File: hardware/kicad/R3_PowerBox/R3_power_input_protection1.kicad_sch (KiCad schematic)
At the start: 13 parts, among them J1 SERVICE / BENCH INPUT 6-12V, Q1 DMP3010LSS-13

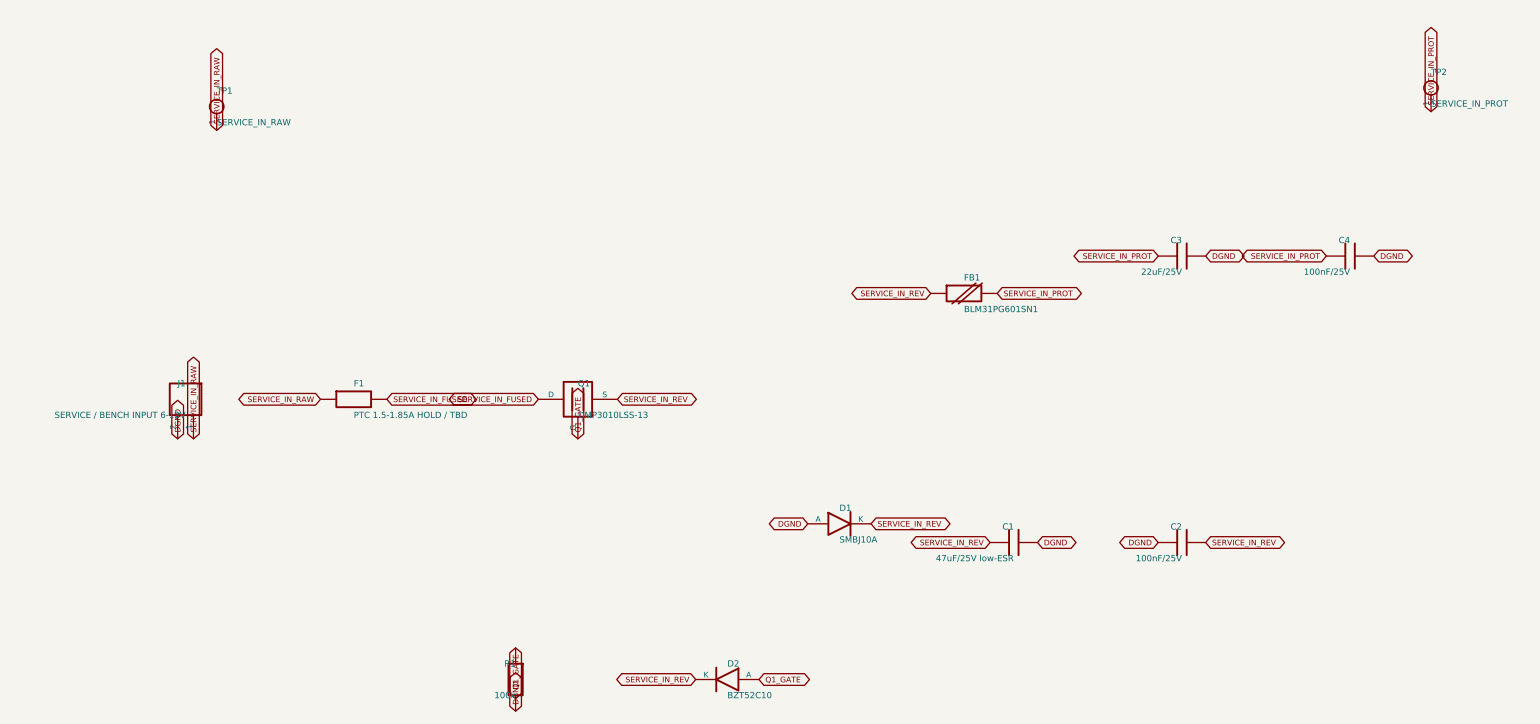
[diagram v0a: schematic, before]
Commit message: Finalize R3 PowerBox pre-placement corrections
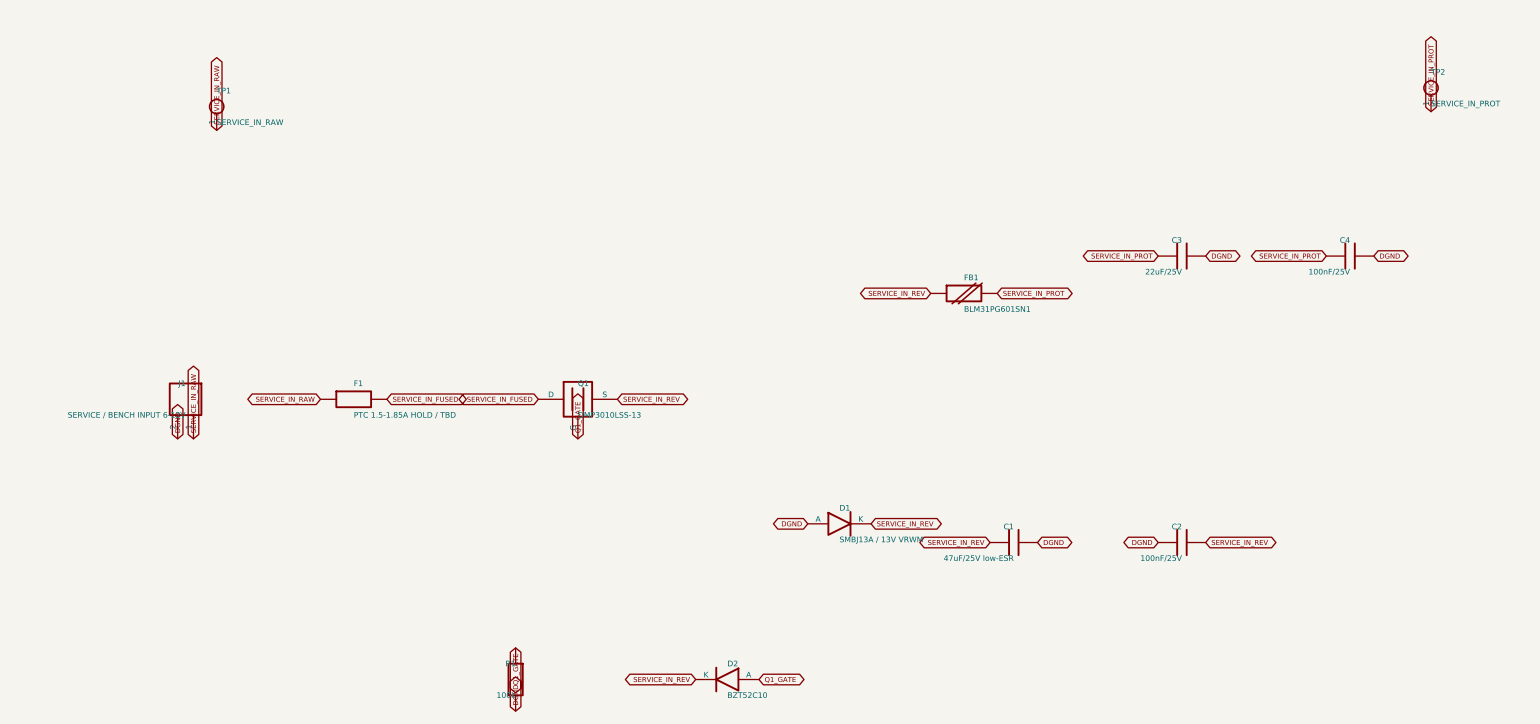
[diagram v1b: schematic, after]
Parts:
- D1: value SMBJ10A -> SMBJ13A / 13V VRWM
